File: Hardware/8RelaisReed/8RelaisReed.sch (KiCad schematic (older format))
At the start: 29 parts, among them J1 ISP, P1 5VIN, P10 CONN_01X02, P11 CONN_01X02, P4 CONN_01X02, P5 CONN_01X02, P6 CONN_01X02, P7 CONN_01X02, P8 CONN_01X02, P9 CONN_01X02, SW1 SW_DPST, SW2 FLASH, U1 AMS1117, U2 ESP-12F, U3 74HCT595, U4 ULN2803A

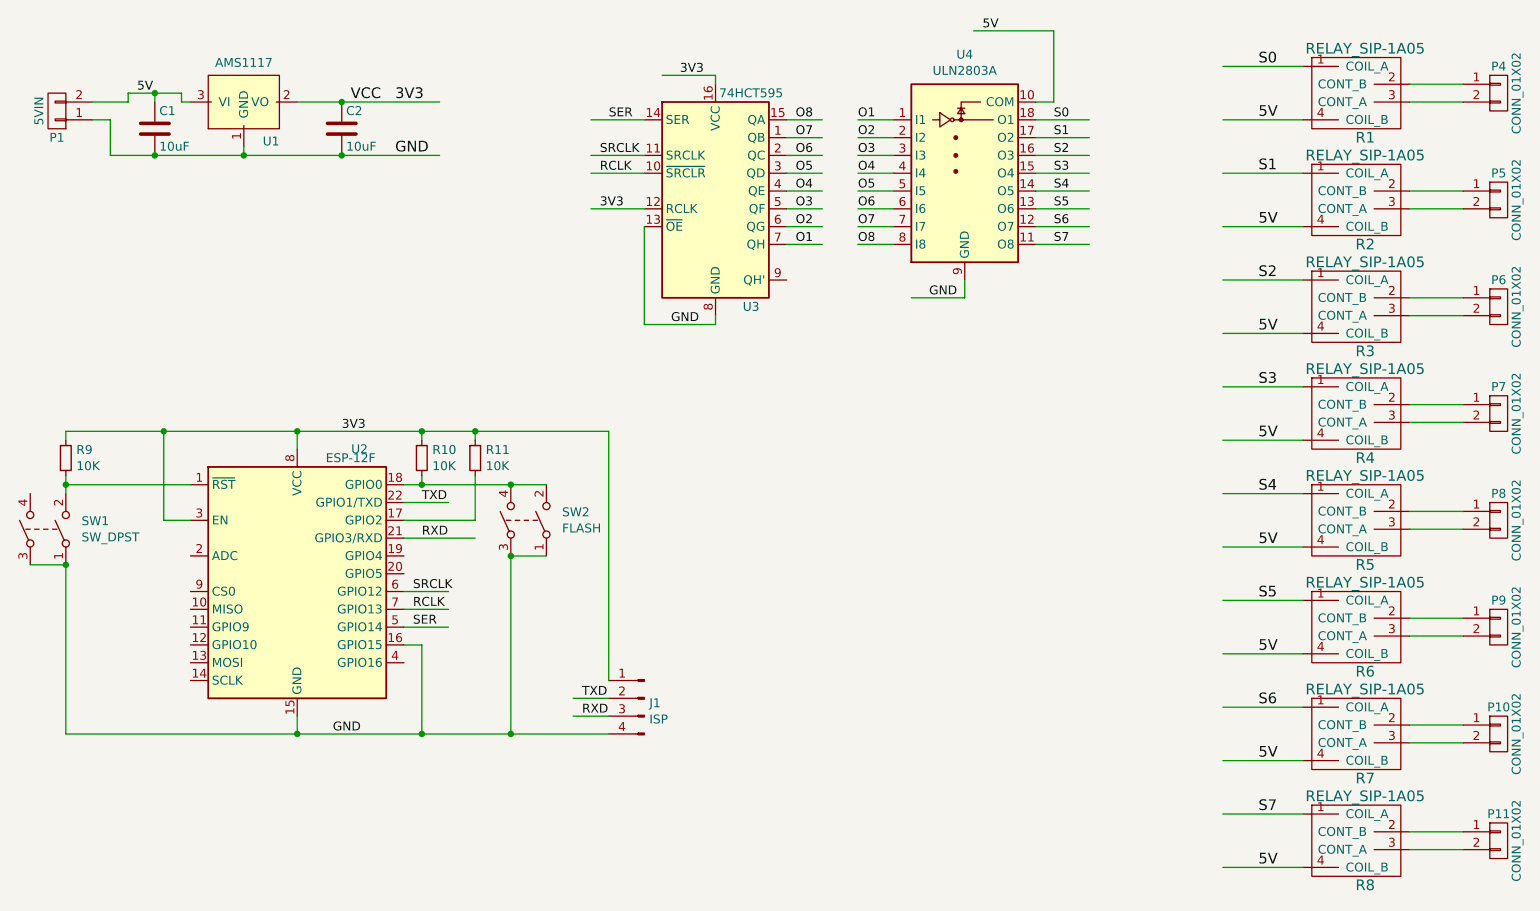
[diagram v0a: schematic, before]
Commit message: Fix on the BaseBoard class
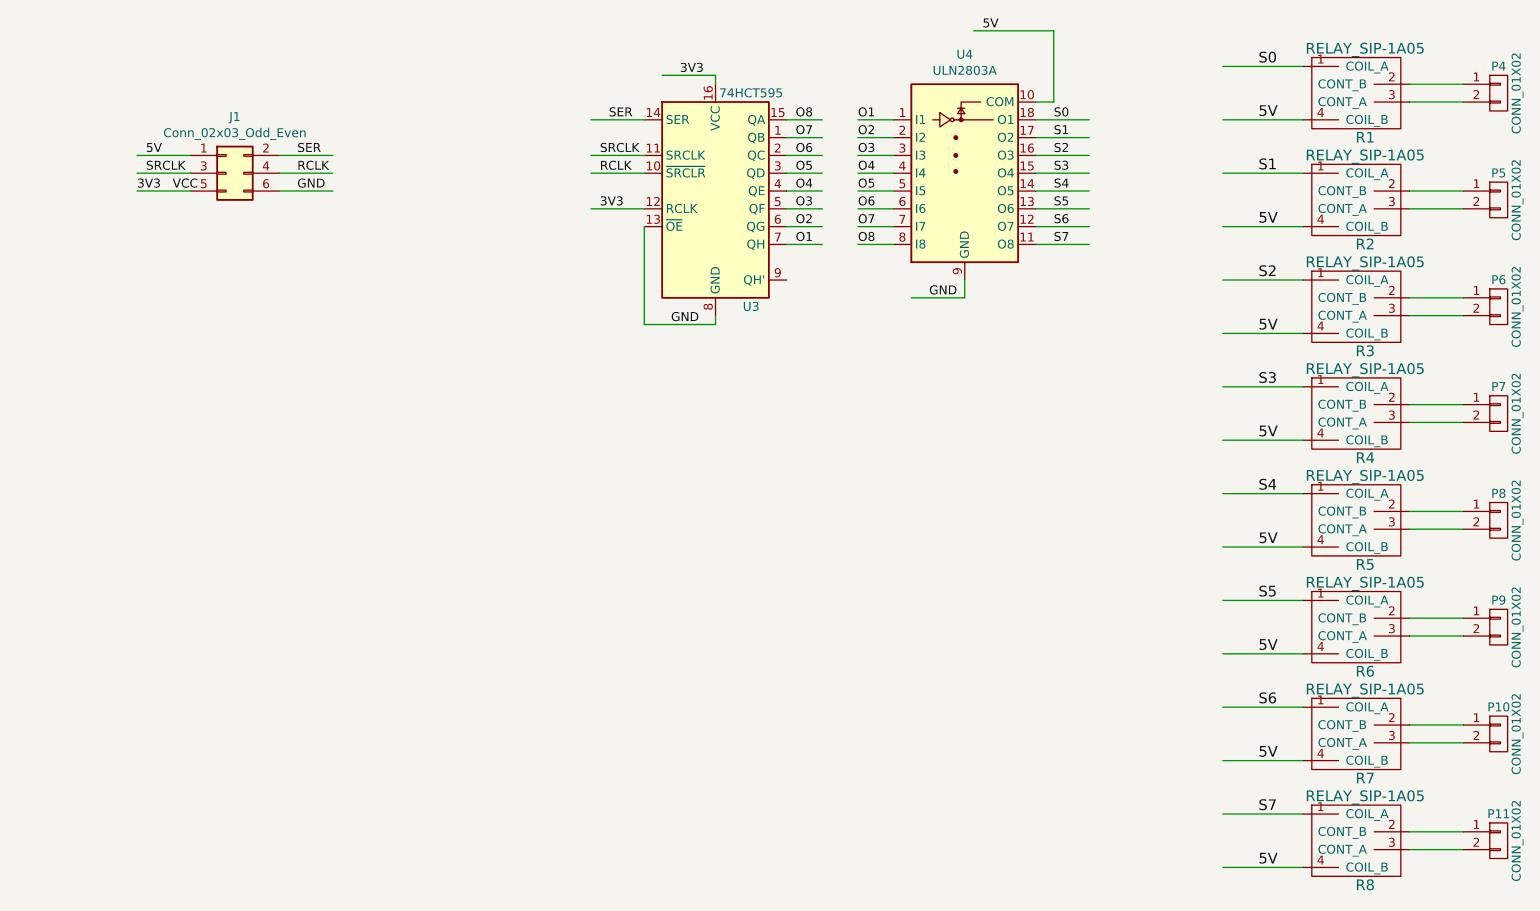
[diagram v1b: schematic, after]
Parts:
- removed C1, C2: 10uF, Capacitor_SMD:C_0805_2012Metric_Pad1.15x1.40mm_HandSolder, symbol 8RelaisReed-rescue:C-mySensors_8RelaisReed-rescue
- removed J1: ISP, Connector_PinHeader_2.54mm:PinHeader_1x04_P2.54mm_Vertical, symbol Connector:Conn_01x04_Male
- removed P1: 5VIN, Connectors:bornier2, symbol 8RelaisReed-rescue:CONN_01X02-mySensors_8RelaisReed-rescue
- removed R10, R11, R9: 10K, Resistor_SMD:R_0805_2012Metric_Pad1.15x1.40mm_HandSolder, symbol Device:R_Small
- removed SW1: SW_DPST, Button_Switch_SMD:SW_SPST_EVPBF, symbol Switch:SW_DPST
- removed SW2: FLASH, Button_Switch_SMD:SW_SPST_EVPBF, symbol Switch:SW_DPST
- removed U1: AMS1117, TO_SOT_Packages_SMD:SOT-223, symbol 8RelaisReed-rescue:AMS1117-mySensors_8RelaisReed-rescue
- removed U2: ESP-12F, RF_Module:ESP-12E, symbol RF_Module:ESP-12F
- added J1: Conn_02x03_Odd_Even, Connector_PinHeader_2.54mm:PinHeader_2x03_P2.54mm_Vertical, symbol Connector_Generic:Conn_02x03_Odd_Even
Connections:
- net labels removed: RXD, TXD
- wire segments 125 -> 76
